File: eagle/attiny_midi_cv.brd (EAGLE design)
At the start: 100 x 80 mm, 29 parts, among them IC1 TL072P, Q518 2N3904, U2 TINY45-20-DIP

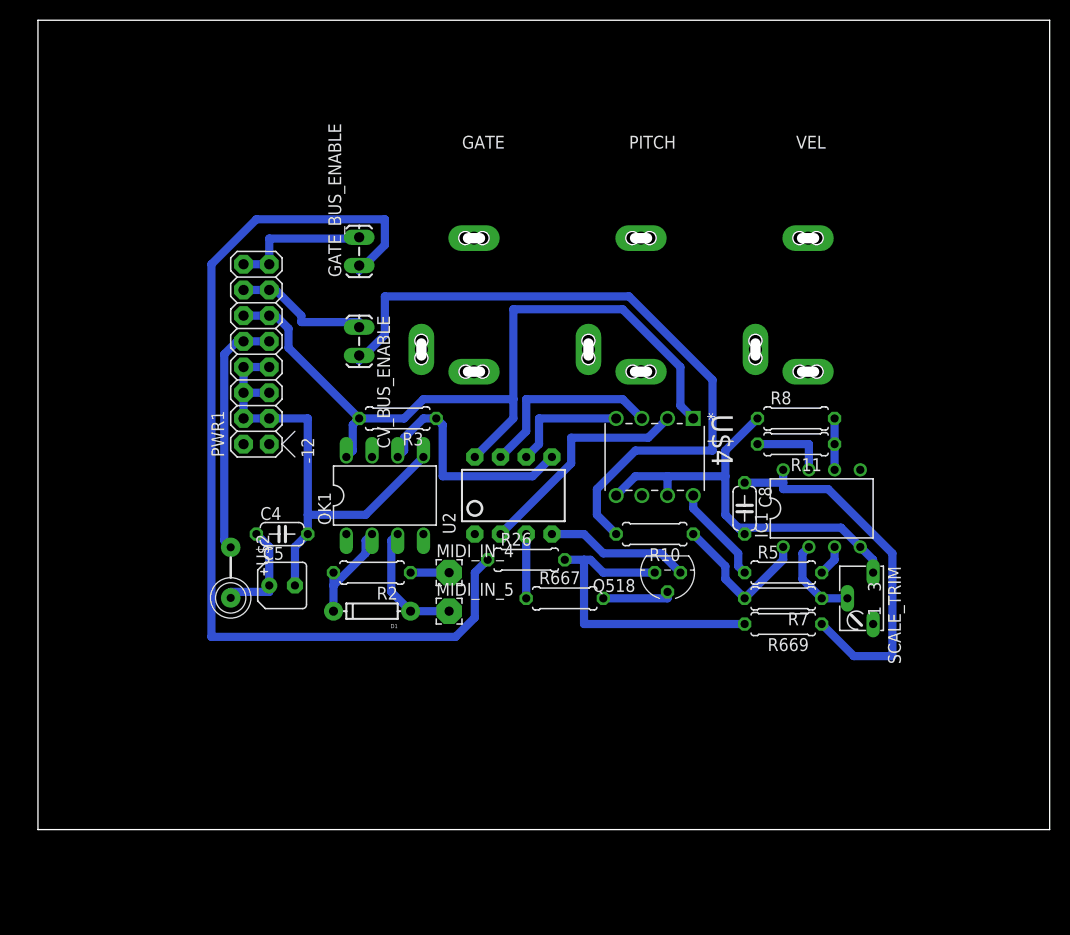
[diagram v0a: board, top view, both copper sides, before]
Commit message: routed
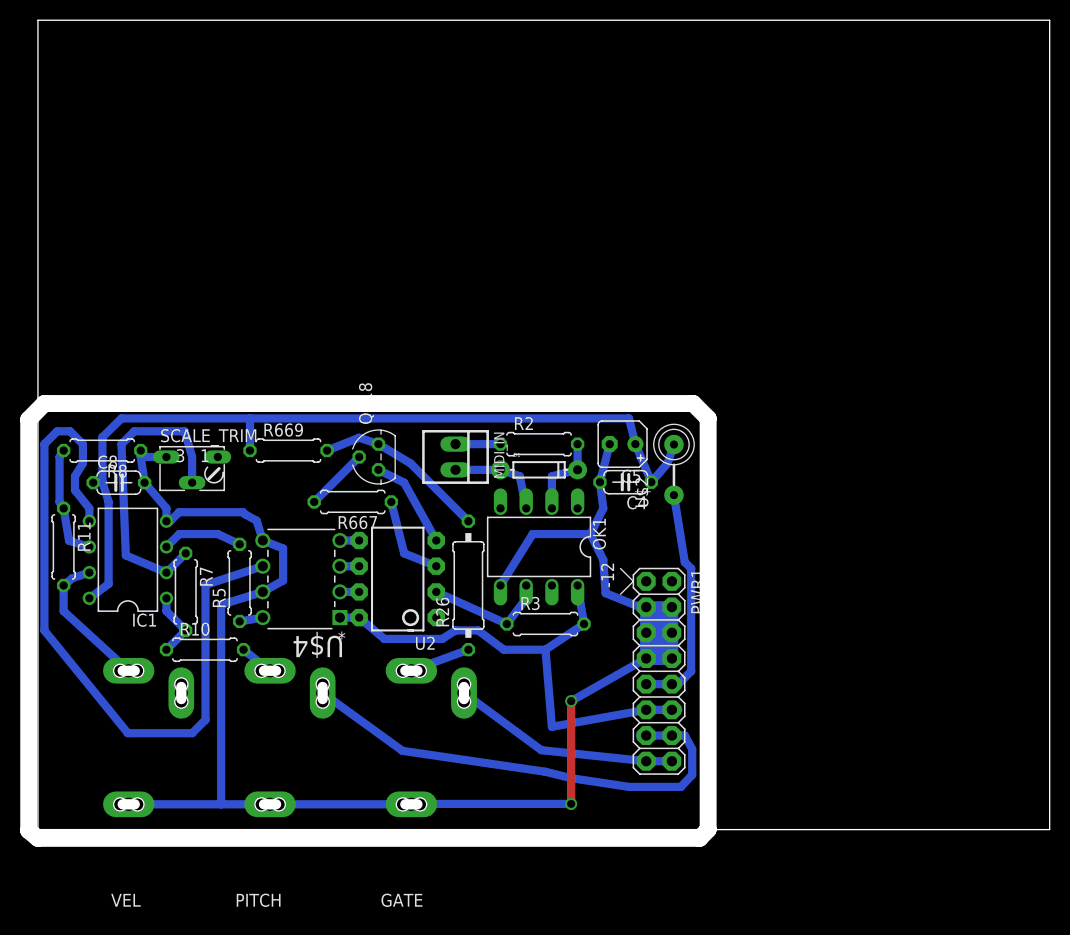
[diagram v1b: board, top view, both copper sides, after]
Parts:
- removed CV_BUS_ENABLE, GATE_BUS_ENABLE: M02LOCK_LONGPADS, SparkFun-Connectors:1X02_LOCK_LONGPADS
- removed MIDI_IN_4: midi pin 4, wirepad:2,54/0,9
- removed MIDI_IN_5: midi pin 5, wirepad:2,54/0,9
- added MIDI_IN: 22-23-2021, con-molex:22-23-2021
- R26: device rcl:0207/7 -> rcl:0309/12
- moved VEL 83.6 mm to (14.0, 0.00), turned to 180 degrees
- moved R11 73.1 mm to (2.54, 27.9), turned to 270 degrees
- moved IC1 68.8 mm to (8.89, 26.7), turned to 90 degrees
- moved SCALE_TRIM 68.7 mm to (15.2, 36.8), turned to 0 degrees
- moved R8 68.7 mm to (6.35, 37.5), turned to 180 degrees
- moved PITCH 66.5 mm to (27.9, 0.00), turned to 180 degrees
- moved C8 61.9 mm to (8.00, 34.3), turned to 0 degrees
- moved GATE 61.1 mm to (41.9, 0.00), turned to 180 degrees
- moved R7 59.1 mm to (14.6, 23.5), turned to 270 degrees
- moved R5 53.7 mm to (19.9, 24.4), turned to 90 degrees
- moved R669 51.8 mm to (24.8, 37.5), turned to 0 degrees
- moved PWR1 47.7 mm to (61.4, 18.2), turned to 270 degrees
- moved R10 45.9 mm to (16.5, 17.8), turned to 0 degrees
- moved U$2 45.0 mm to (62.9, 35.6), turned to 90 degrees
- moved C5 36.4 mm to (57.8, 38.1), turned to 180 degrees
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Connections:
- removed net N$1: GATE_BUS_ENABLE.2, PWR1.15, PWR1.16
- removed net N$9: CV_BUS_ENABLE.2, PITCH.P$3, R10.2
- new net N$4: GATE.P$3, R26.1
- new net N$5: PITCH.P$3, R10.2
- net N$15: now also PITCH.P$2; no longer CV_BUS_ENABLE.1
- net N$25: now also U2.6; no longer U2.7
- net N$26: now also U2.5; no longer U2.6
- net N$3: now also MIDI_IN.2; no longer MIDI_IN_5.1
- net N$30: now also U2.2; no longer U2.5
- net N$31: now also GATE.P$2, PWR1.15, PWR1.16; no longer GATE.P$3, GATE_BUS_ENABLE.1, R26.1
- net N$45: now also U2.7; no longer U2.2
- net N$8: now also MIDI_IN.1; no longer MIDI_IN_4.1
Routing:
- net N$31: track 95.5 -> 22.5 mm
- net N$14: track 0.00 -> 72.2 mm
- net N$10: track 90.3 -> 160.3 mm, vias 0 -> 2
- net N$9: track 68.9 -> 0.00 mm
- net +12V: track 48.2 -> 85.0 mm
- net N$15: track 13.6 -> 47.7 mm
- net +5V: track 77.8 -> 50.7 mm
- net N$12: track 8.67 -> 30.0 mm
- net N$45: track 22.7 -> 1.91 mm
- net N$25: track 19.0 -> 1.91 mm
- net N$20: track 31.6 -> 17.2 mm
- net N$1: track 14.1 -> 0.00 mm
- net N$30: track 23.7 -> 12.1 mm
- net N$26: track 12.0 -> 1.91 mm
- net N$27: track 15.1 -> 6.66 mm
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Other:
- board size 100 x 80 mm -> 100.9 x 80.9 mm
